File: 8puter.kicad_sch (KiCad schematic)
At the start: 2 parts

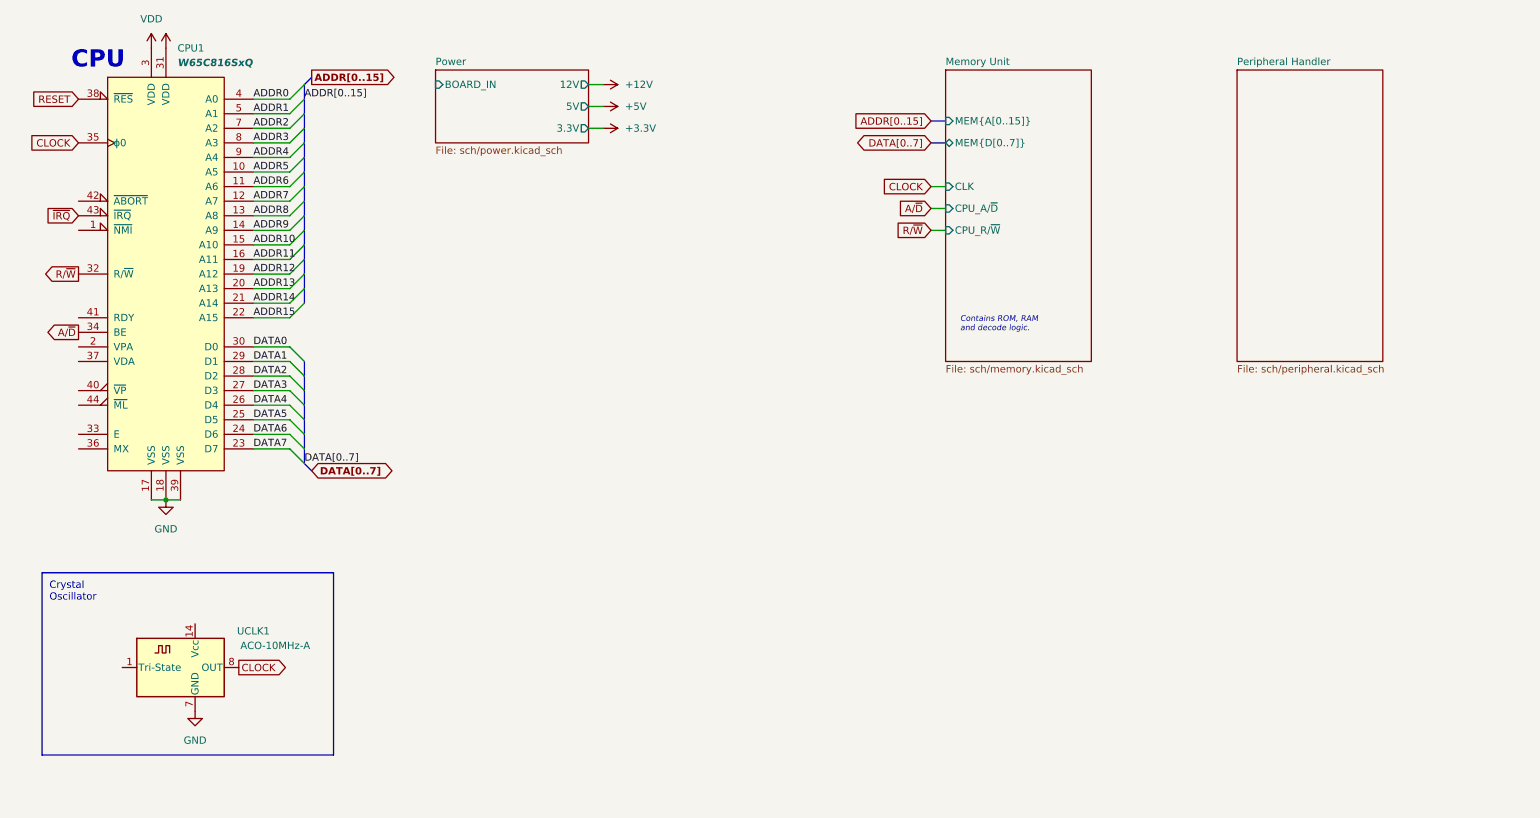
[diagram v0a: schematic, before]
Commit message: Bus control
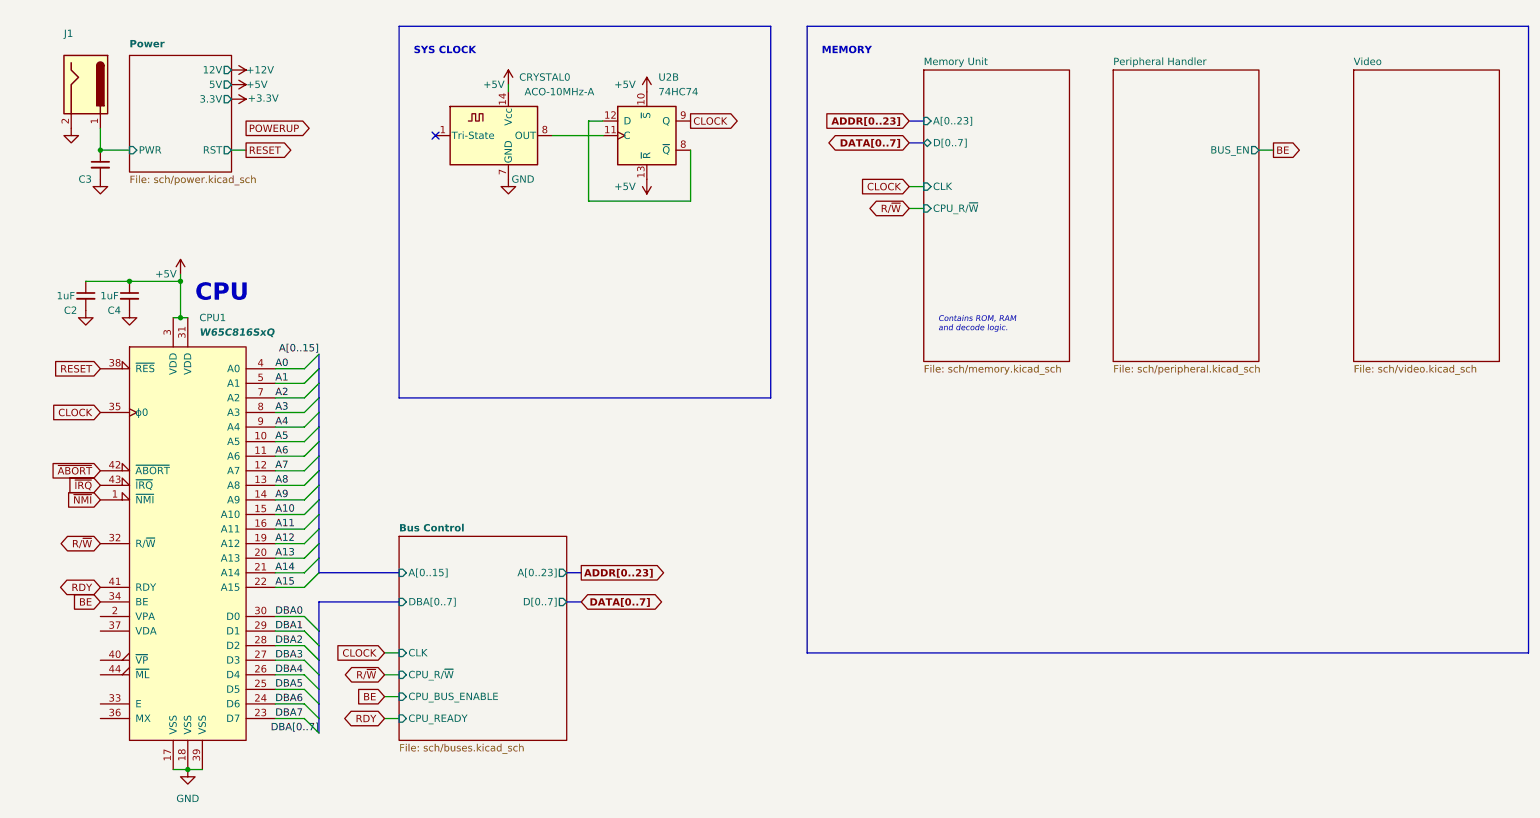
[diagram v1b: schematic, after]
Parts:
- added C2, C4: 1uF, symbol Device:C_Small
- added C3: (no value), symbol Device:C_Small
- added J1: (no value), symbol Connector:Jack-DC
- added U2: 74HC74, symbol 74xx:74LS74
- CPU1: footprint Package_QFP:PQFP-44_10x10mm_P0.8mm -> Package_DIP:DIP-40_W25.4mm_Socket_LongPads
- renumbered UCLK1 to CRYSTAL0
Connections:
- net VDD is gone; now on net +5V: CPU1.3 (VDD), CPU1.31 (VDD)
- net +5V: now also CRYSTAL0.14 (Vcc), C2.1, C4.1, U2.10 (~{S}), U2.13 (~{R})
- net CLOCK: now also U2.9 (Q); no longer CRYSTAL0.8 (OUT)
- net GND: now also C2.2, C3.2, C4.2, J1.2
- net ~{NMI}: now reaches CPU1.1 (~{NMI})
- net RDY: now reaches CPU1.41 (RDY)
- net ~{ABORT}: now reaches CPU1.42 (~{ABORT})
- net ADDR0 renamed A0
- net ADDR1 renamed A1
- net ADDR10 renamed A10
- net ADDR11 renamed A11
- net ADDR12 renamed A12
- net ADDR13 renamed A13
- net ADDR14 renamed A14
- net ADDR15 renamed A15
- net ADDR2 renamed A2
- net ADDR3 renamed A3
- net ADDR4 renamed A4
- net ADDR5 renamed A5
- net ADDR6 renamed A6
- net ADDR7 renamed A7
- net ADDR8 renamed A8
- net ADDR9 renamed A9
- net A/~{D} renamed BE
- net DATA0 renamed DBA0
- net DATA1 renamed DBA1
- net DATA2 renamed DBA2
- net DATA3 renamed DBA3
- net DATA4 renamed DBA4
- net DATA5 renamed DBA5
- net DATA6 renamed DBA6
- net DATA7 renamed DBA7
- new net: CRYSTAL0.8 (OUT), U2.11 (C)
- new net: U2.12 (D), U2.8 (~{Q})
- new net Power/PWR: C3.1, J1.1
- no-connect marks 0 -> 1
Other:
- added sheet Bus Control (sch/buses.kicad_sch)
- added sheet Video (sch/video.kicad_sch)
- sheet Memory Unit ports: added A[0..23], D[0..7]; removed CPU_A/~{D}, MEM{A[0..15]}, MEM{D[0..7]}
- sheet Peripheral Handler ports: added BUS_EN; removed none
- sheet Power ports: added PWR, RST; removed BOARD_IN
- note added: "MEMORY"
- note added: "SYS CLOCK"
- note removed: "Crystal Oscillator"
- moved on the sheet: CPU1, CRYSTAL0
